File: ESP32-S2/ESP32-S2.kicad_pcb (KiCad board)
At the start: 2 copper layers, 27.9 x 70 mm, 39 parts, among them J1 Conn_01x18_Male, J2 Conn_01x21_Male, J3 USB_A, J4 TYPE-C-31-M-12, Q2 L8050QLT1G, Q3 L8050QLT1G, SW1 EN/RESET, SW2 BOOT/SELECT, U2 ESP32-S2-WROOM-ESP32-S2-WROOM, U3 AMS1117-3.3, U4 CH340C

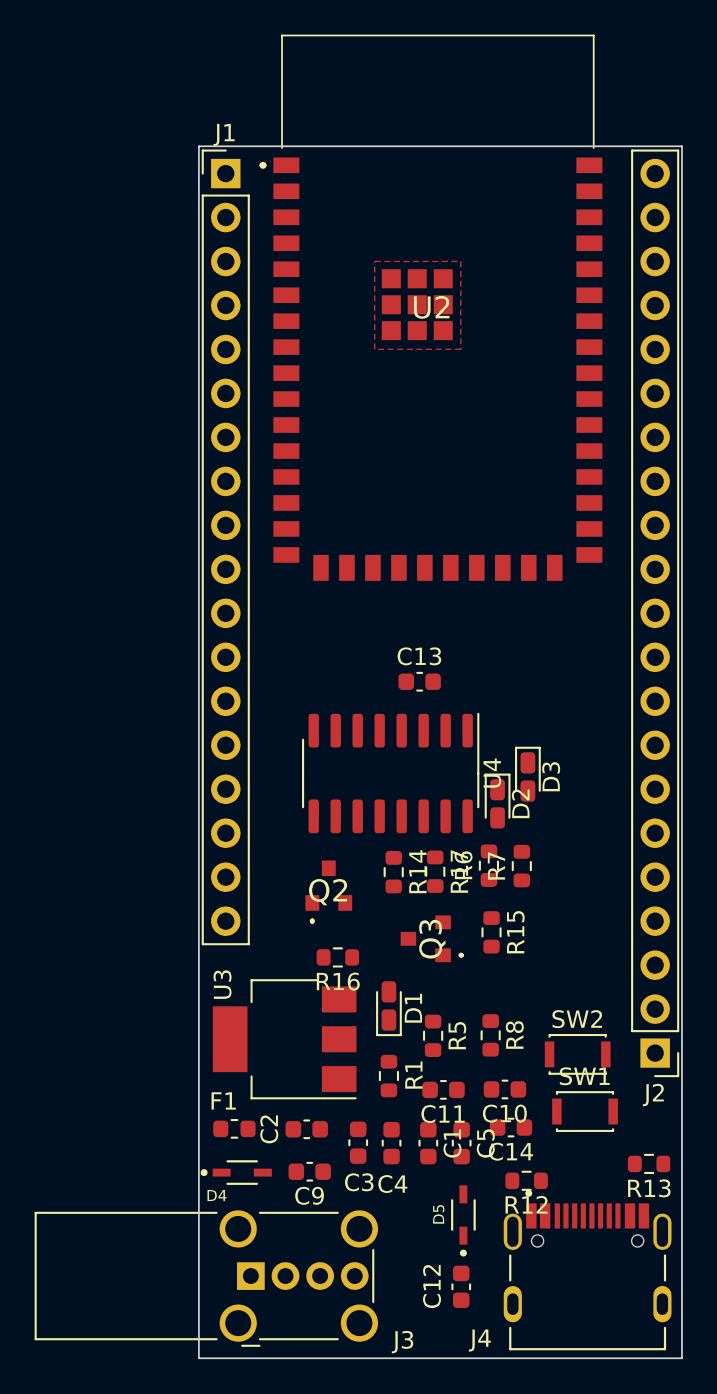
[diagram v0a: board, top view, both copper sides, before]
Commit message: routing done- v.1
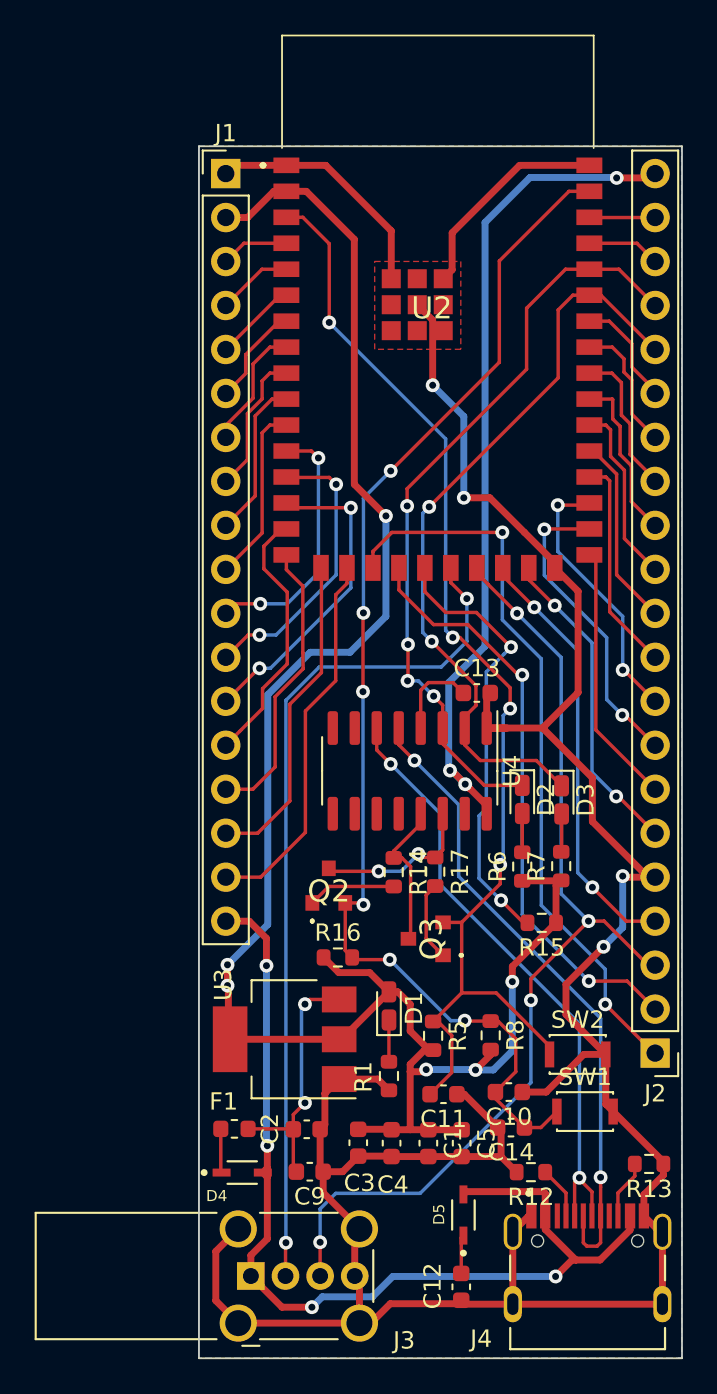
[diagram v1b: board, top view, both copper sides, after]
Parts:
- moved C13 3.36 mm to (152.9, 98.7)
- moved R15 2.95 mm to (156.7, 112.0), turned to 180 degrees
- moved D3 2.36 mm to (157.8, 104.8)
- moved R7 2.27 mm to (157.8, 108.7)
- moved R6 1.93 mm to (155.6, 108.7)
- moved D2 1.45 mm to (155.6, 104.8)
- moved U4 1.11 mm to (149.1, 103.2)
- moved R12 0.56 mm to (156.1, 126.3)
- moved C10 0.27 mm to (154.8, 121.7)
- moved C11 0.25 mm to (151.0, 121.8)
- turned R1 to 270 degrees
- turned R16 to 0 degrees
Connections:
- J1 pad 2: /3V3 -> +3V3
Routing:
- net GND: track 0.00 -> 184.8 mm, vias 0 -> 4
- net +3V3: track 0.00 -> 115.0 mm, vias 0 -> 6
- net /CHIP_PU: track 0.00 -> 72.4 mm, vias 0 -> 6
- net /GPIO0: track 0.00 -> 67.7 mm, vias 0 -> 4
- net /GPIO20: track 0.00 -> 57.8 mm, vias 0 -> 4
- net /VBUS: track 0.00 -> 57.6 mm, vias 0 -> 4
- net /GPIO19: track 0.00 -> 49.8 mm, vias 0 -> 2
- net VCC: track 0.00 -> 48.9 mm, vias 0 -> 3
- net /RXD0: track 0.00 -> 44.1 mm, vias 0 -> 4
- net /TXD0: track 0.00 -> 43.7 mm, vias 0 -> 2
- net /GPIO16: track 0.00 -> 42.6 mm, vias 0 -> 2
- net /DP1: track 0.00 -> 37.3 mm, vias 0 -> 2
- net /DN1: track 0.00 -> 35.6 mm, vias 0 -> 2
- net /GPIO17: track 0.00 -> 34.2 mm, vias 0 -> 2
- net /GPIO18: track 0.00 -> 25.7 mm, vias 0 -> 2
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- added copper zone on B.Cu, net GND
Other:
- net class Default: trace_width 0.4 -> 0.2
